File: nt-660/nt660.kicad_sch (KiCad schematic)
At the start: 156 parts, among them J1 USB_mini_micro_B, J2 ISP, K1 KEYSW, K10 KEYSW, K11 KEYSW, K12 KEYSW, K13 KEYSW, K14 KEYSW, K15 KEYSW, K16 KEYSW, K17 KEYSW, K18 KEYSW, K19 KEYSW, K2 KEYSW, K20 KEYSW, K21 KEYSW, K22 KEYSW, K23 KEYSW, K24 KEYSW, K25 KEYSW, K26 KEYSW, K27 KEYSW, K28 KEYSW, K29 KEYSW, K3 KEYSW, K30 KEYSW, K31 KEYSW, K32 KEYSW, K33 KEYSW, K34 KEYSW, K35 KEYSW, K36 KEYSW, K37 KEYSW, K38 KEYSW, K39 KEYSW, K4 KEYSW, K40 KEYSW, K41 KEYSW, K42 KEYSW, K43 KEYSW, K44 KEYSW, K44-1 KEYSW, K46 KEYSW, K46-1 KEYSW, K47 KEYSW, K48 KEYSW, K49 KEYSW, K5 KEYSW, K50 KEYSW, K51 KEYSW, K52 KEYSW, K53 KEYSW, K54 KEYSW, K55 KEYSW, K56 KEYSW, K57 KEYSW, K58 KEYSW, K59 KEYSW, K6 KEYSW, K61 KEYSW, K62 KEYSW, K63 KEYSW, K67 KEYSW, K7 KEYSW, K70 KEYSW, K71 KEYSW, K72 KEYSW, K73 KEYSW, K74 KEYSW, K75 KEYSW, K8 KEYSW, K9 KEYSW, SW1 Reset, U1 ATmega32U4, U2 USBLC6-2SC6, X1 CSTNE16M0V530000R0

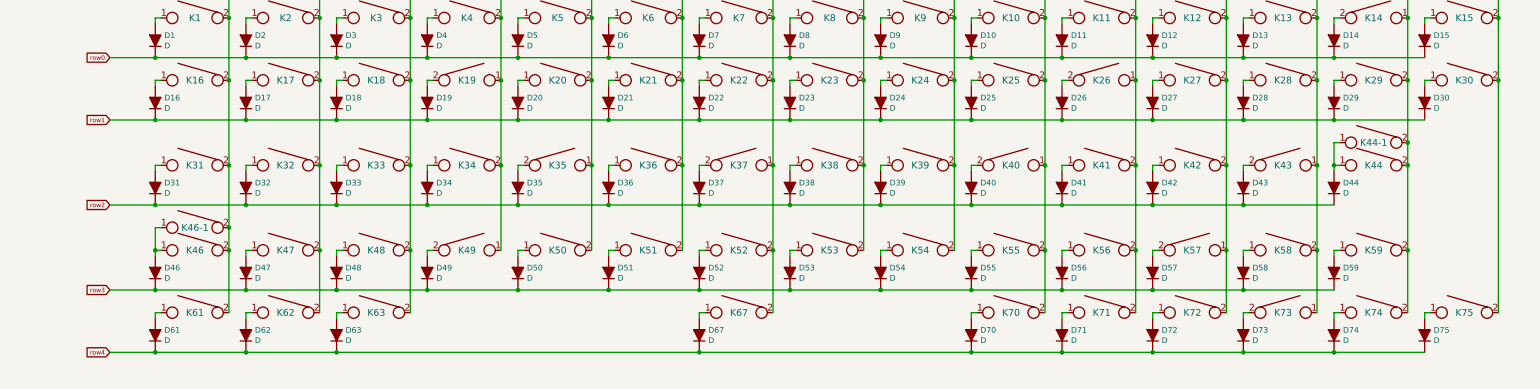
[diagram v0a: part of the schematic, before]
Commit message: nt-660 rev1.1
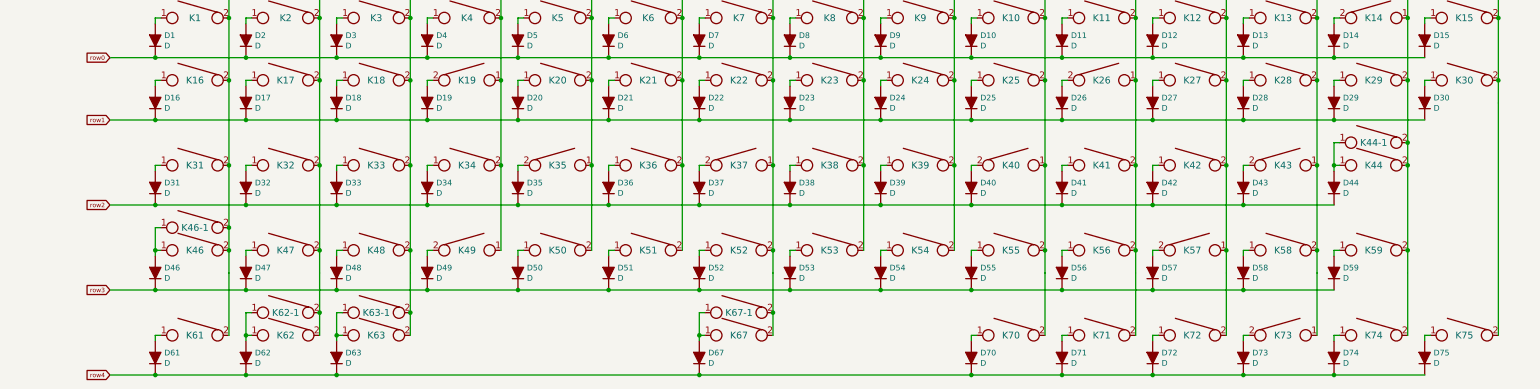
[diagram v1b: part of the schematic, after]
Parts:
- added K62-1, K63-1: KEYSW, Keeb_switches:CHERRY_PLATE_125H, symbol keyboard_parts:KEYSW
- added K67-1: KEYSW, Keeb_switches:CHERRY_PCB_600C_H_F, symbol keyboard_parts:KEYSW
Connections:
- net col1: now also K62-1.2
- net col2: now also K63-1.2
- net col6: now also K67-1.2
- net at D63.2 (A), K63.1: now also K63-1.1
- net at D62.2 (A), K62.1: now also K62-1.1
- net at D67.2 (A), K67.1: now also K67-1.1
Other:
- moved on the sheet: D61, D62, D63, D67, D70, D71, D72, D73, D74, D75, K61, K62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
